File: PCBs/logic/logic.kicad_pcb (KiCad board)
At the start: 2 copper layers, 149.5 x 111.5 mm, 7 parts, among them J1 PWR_Conn, J2 Conn_01x04, U8 ESP32-C6-DEVKITC-1-N8

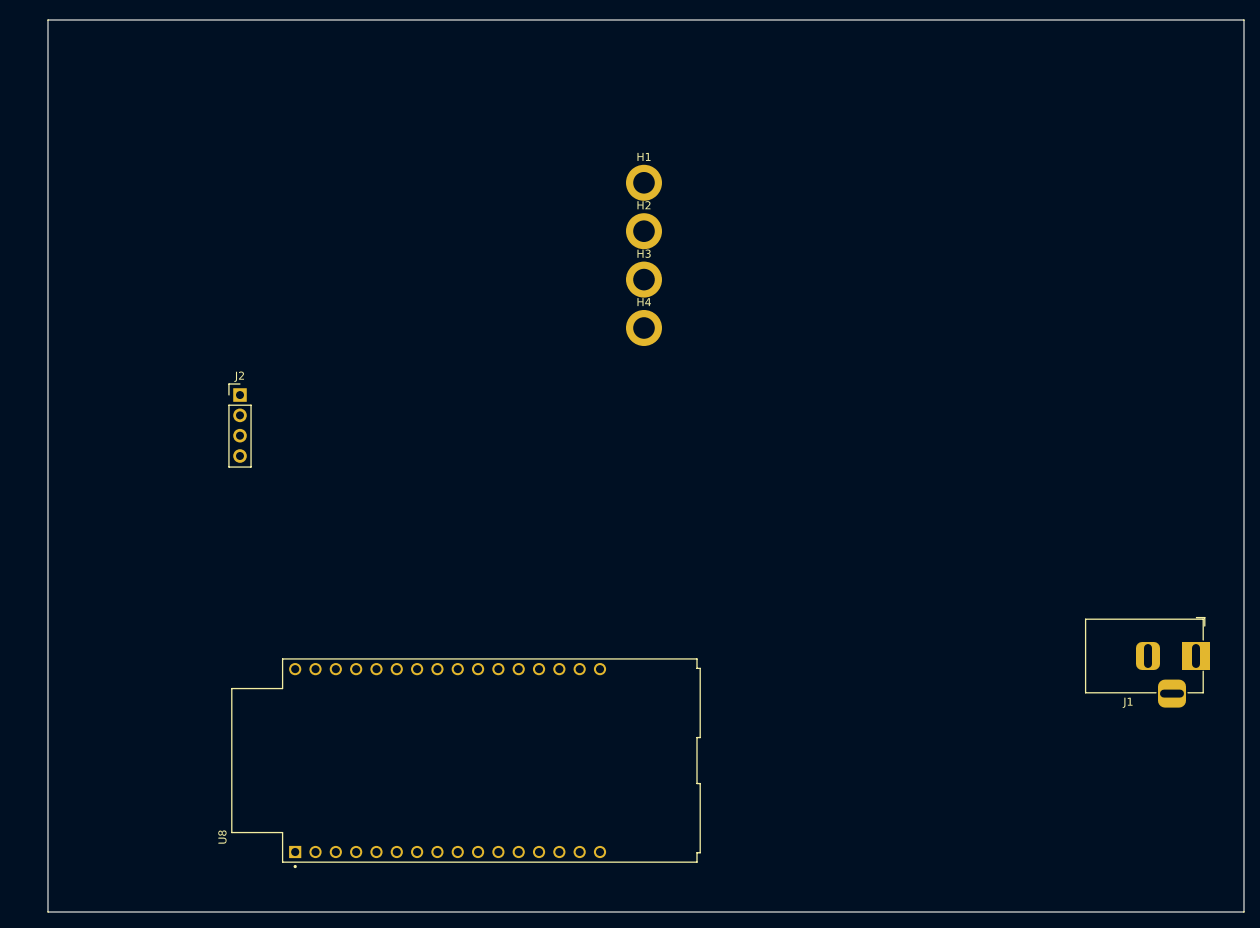
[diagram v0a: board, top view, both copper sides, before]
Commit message: Logic PCB finished
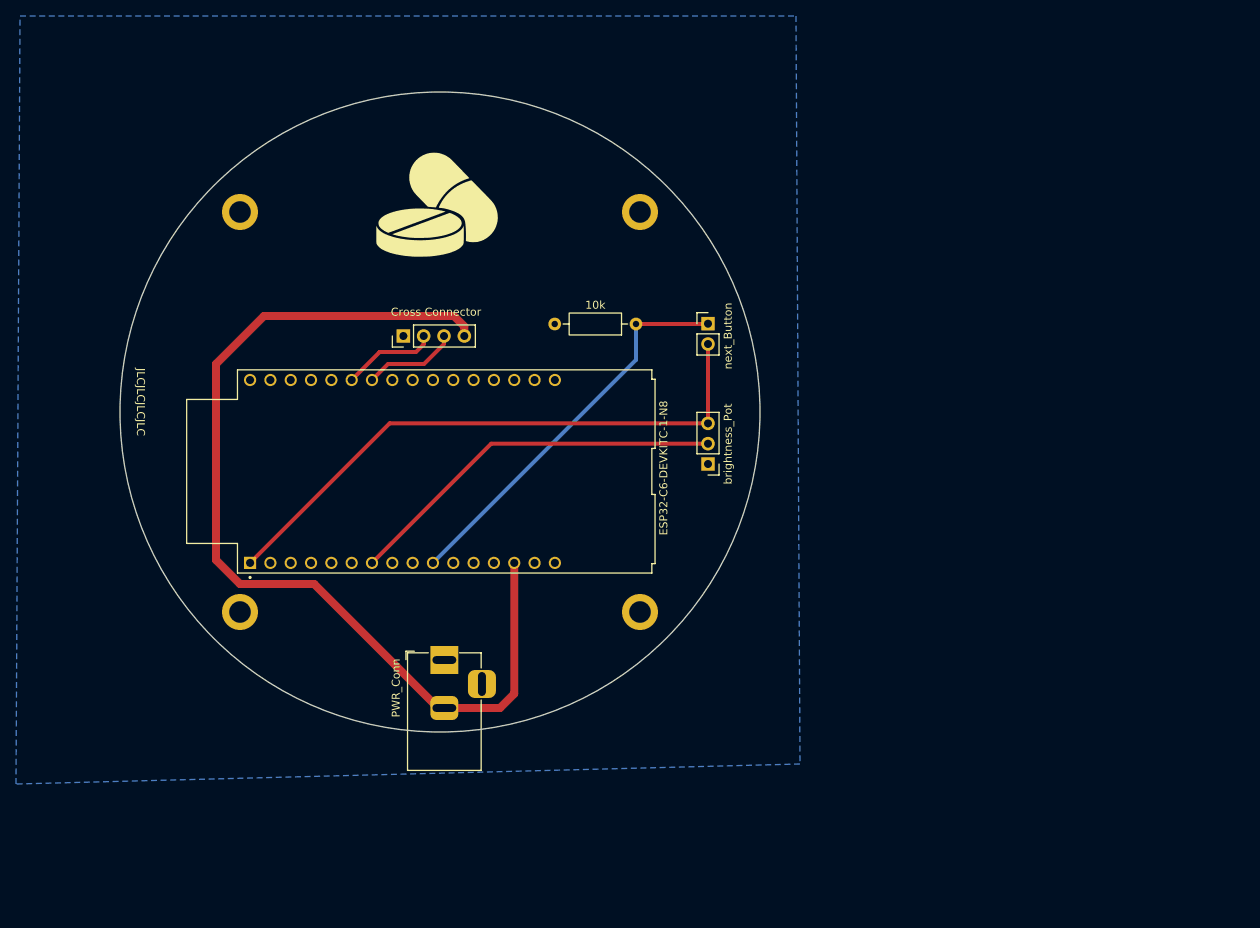
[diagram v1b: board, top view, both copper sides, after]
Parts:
- added G***: LOGO, LOGO, F.Cu at (149.6, 74.1)
- added G***: LOGO, LOGO, B.Cu at (150.0, 74.0)
- added R1: 10k, Resistor_THT:R_Axial_DIN0207_L6.3mm_D2.5mm_P10.16mm_Horizontal, F.Cu at (174.5, 89.0)
- added RV1: brightness_Pot, Connector_PinHeader_2.54mm:PinHeader_1x03_P2.54mm_Vertical, F.Cu at (183.5, 106.5)
- added SW1: next_Button, Connector_PinHeader_2.54mm:PinHeader_1x02_P2.54mm_Vertical, F.Cu at (183.5, 89.0)
- J2: value Conn_01x04 -> Cross Connector
- moved J1 94.0 mm to (150.5, 131.0), turned to 90 degrees
- moved H4 61.7 mm to (125.0, 125.0)
- moved H1 50.6 mm to (125.0, 75.0)
- moved H3 41.6 mm to (175.0, 125.0)
- moved U8 36.6 mm to (150.6, 107.4)
- moved J2 21.7 mm to (145.4, 90.5), turned to 90 degrees
- moved H2 2.45 mm to (175.0, 75.0)
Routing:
- net +5V: track 0.00 -> 121.6 mm
- net +3.3V: track 0.00 -> 74.4 mm
- net /nextPattern: track 0.00 -> 49.4 mm
- net /brightness: track 0.00 -> 48.2 mm
- net /SCL: track 0.00 -> 11.9 mm
- net /SDA: track 0.00 -> 11.9 mm
- added copper zone on B.Cu, net GND
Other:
- board size 149.5 x 111.5 mm -> 80 x 80 mm
- board text added: "JLCJLCJLCJLC"
- board text added: "Logic PCB By Vincent Philippoz 02/2026"
- board text added: "PHARMACY CROSS PROJECT"
